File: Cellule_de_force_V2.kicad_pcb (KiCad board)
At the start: 4 copper layers, 57 x 50.8 mm, 73 parts, among them IC2 TPS61086DRCR, J1 Conn_01x07_Pin, J3 691408720004B, Q1 SI2303CDS-T1-GE3, U1 AD7190WBRUZ, U2 LT3042IMSE, Y2 CSTCR4M91G53-R0

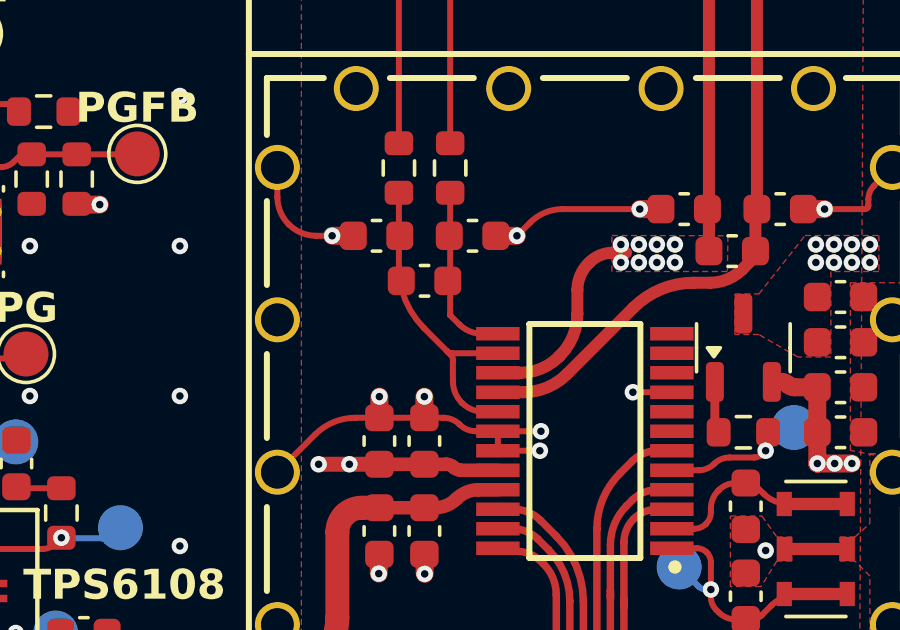
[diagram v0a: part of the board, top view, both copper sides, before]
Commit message: [PCB V4]
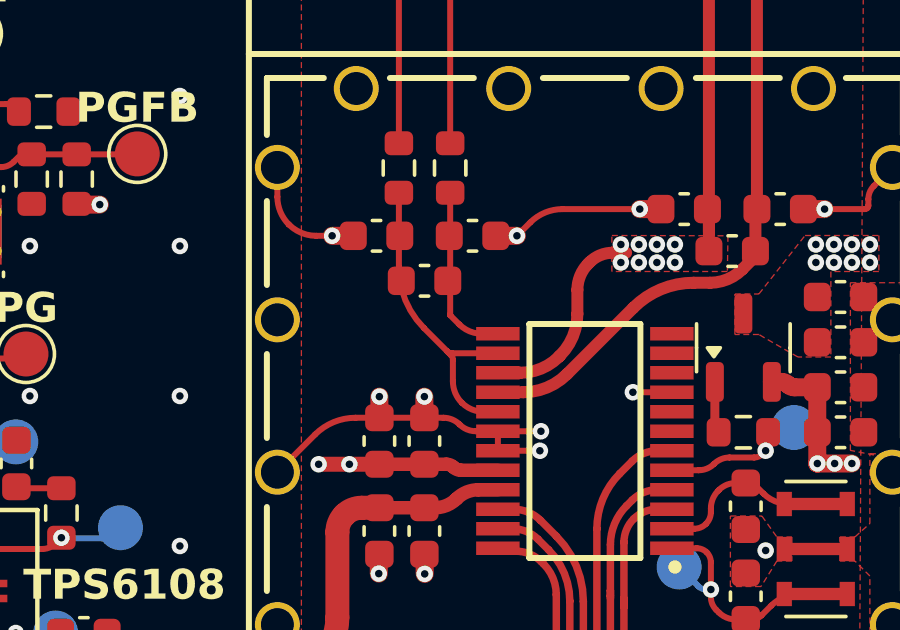
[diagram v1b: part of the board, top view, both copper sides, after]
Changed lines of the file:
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@@
-	)
-	(arc
-		(start 144.005 87.295)
-		(mid 144.002928 87.3)
-		(end 144.005 87.305)
-		(width 0.2)
-		(layer "F.Cu")
-		(net 3)
 	)
 	(arc
